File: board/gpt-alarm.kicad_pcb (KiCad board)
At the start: 2 copper layers, 105 x 64 mm, 12 parts, among them J1 Input, J2 Siren_Out, K1 HK19F-DCxxV-SHC, Q1 AO3400A, Q2 AO3400A

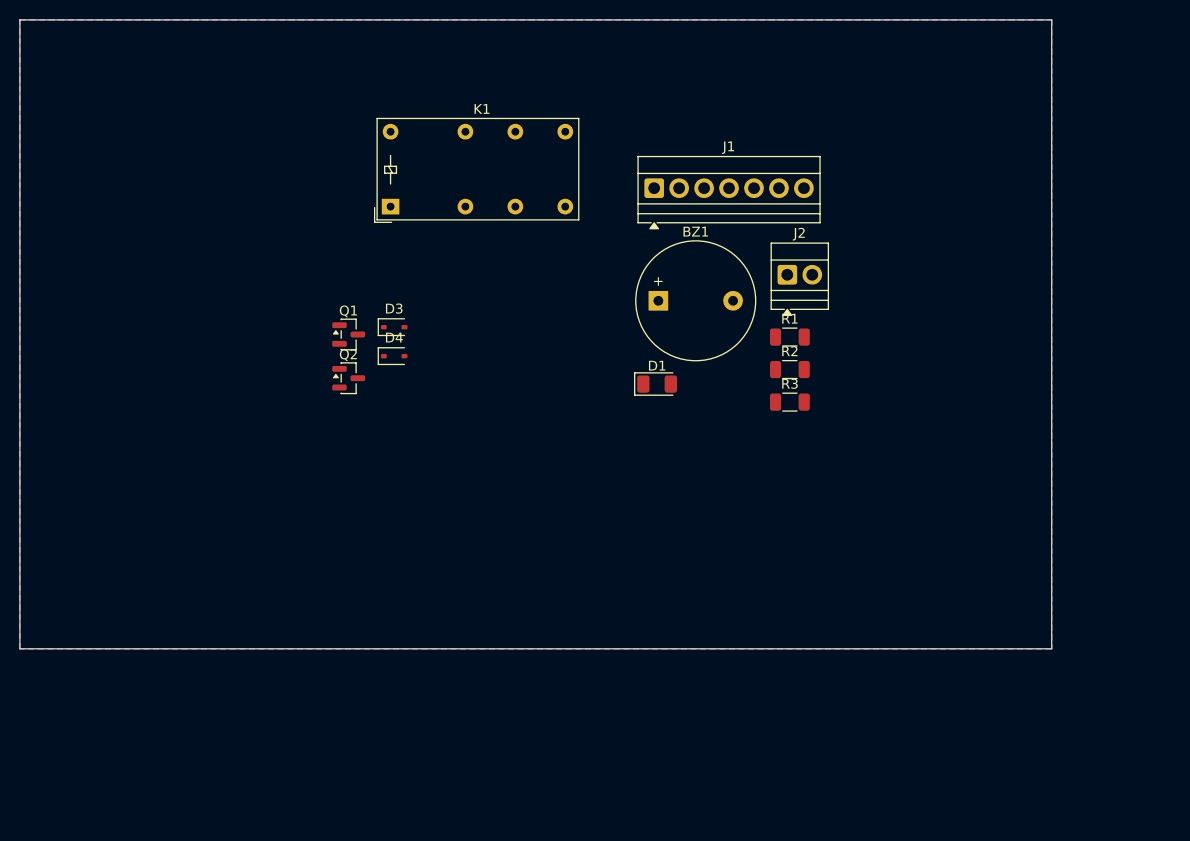
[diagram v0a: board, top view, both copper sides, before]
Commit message: feat: pcb layout
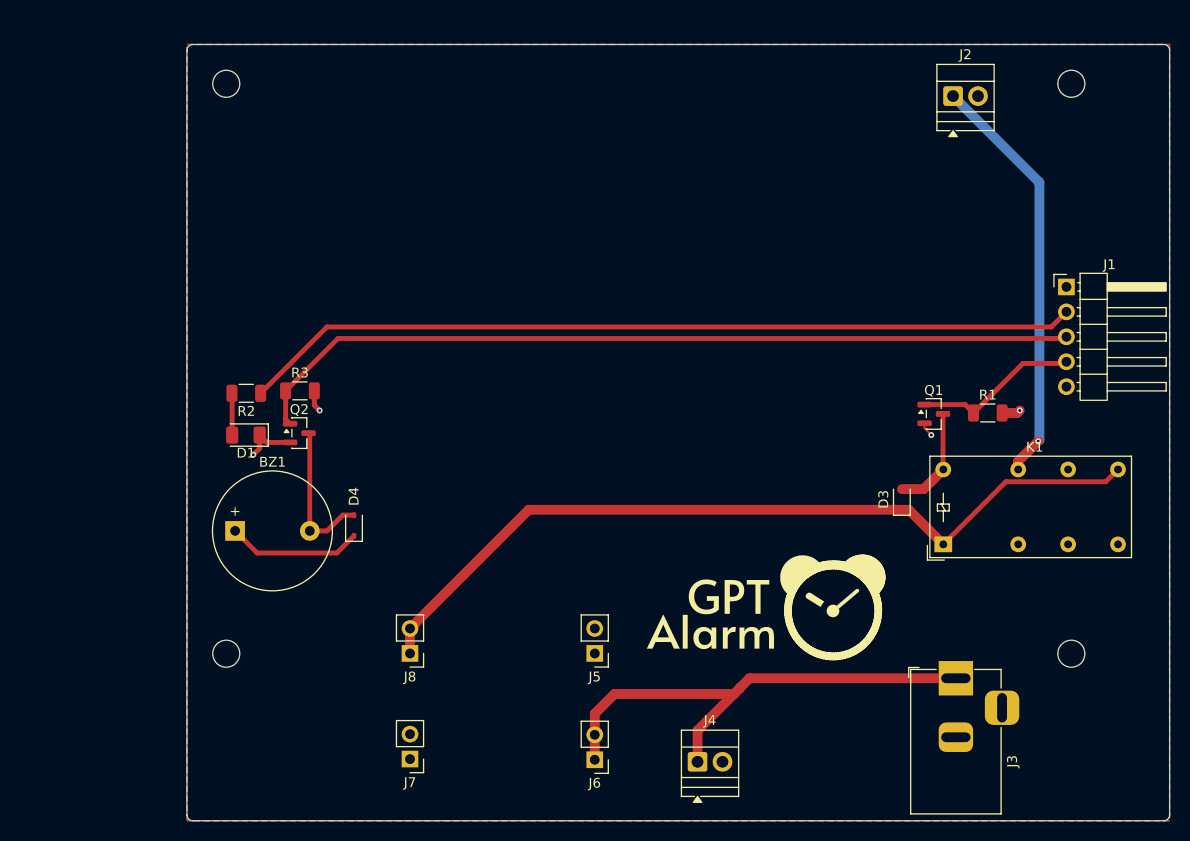
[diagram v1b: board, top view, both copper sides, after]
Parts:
- added J3: 19V IN, Connector_BarrelJack:BarrelJack_Horizontal, F.Cu at (181.8, 105.0)
- added J4: 19V OUT, TerminalBlock:TerminalBlock_Xinya_XY308-2.54-2P_1x02_P2.54mm_Horizontal, F.Cu at (155.5, 113.5)
- added J5: BUCK IN -, Connector_PinHeader_2.54mm:PinHeader_1x02_P2.54mm_Vertical, F.Cu at (145.0, 102.5)
- added J6: BUCK IN +, Connector_PinHeader_2.54mm:PinHeader_1x02_P2.54mm_Vertical, F.Cu at (145.0, 113.3)
- added J7: BUCK OUT -, Connector_PinHeader_2.54mm:PinHeader_1x02_P2.54mm_Vertical, F.Cu at (126.2, 113.2)
- added J8: BUCK OUT +, Connector_PinHeader_2.54mm:PinHeader_1x02_P2.54mm_Vertical, F.Cu at (126.2, 102.5)
- J1: value Input -> Conn_01x05_Pin; footprint TerminalBlock:TerminalBlock_Xinya_XY308-2.54-7P_1x07_P2.54mm_Horizontal -> Connector_PinHeader_2.54mm:PinHeader_1x05_P2.54mm_Horizontal
- moved K1 65.9 mm to (180.5, 91.4)
- moved Q1 60.1 mm to (179.5, 78.1)
- moved R2 55.4 mm to (109.5, 76.0), turned to 180 degrees
- moved D3 54.6 mm to (176.2, 86.8), turned to 90 degrees
- moved R3 49.9 mm to (115.0, 75.8)
- moved BZ1 49.0 mm to (108.4, 90.0)
- moved J1 43.1 mm to (193.0, 65.2)
- moved D1 42.2 mm to (109.5, 80.2), turned to 180 degrees
- moved J2 24.8 mm to (181.5, 45.8)
- moved R1 21.6 mm to (185.0, 78.0)
- moved D4 17.7 mm to (120.5, 89.5), turned to 90 degrees
- moved Q2 7.51 mm to (114.9, 80.0)
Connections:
- J1 pad 1: +12V -> GND
- J1 pad 2: +5V -> Net-(J1-Pin_2)
- J1 pad 3: +3V3 -> /buzz_sig
- J1 pad 5: /buzz_sig -> +5V
- R2 pad 1: Net-(J1-Pin_6) -> Net-(J1-Pin_2)
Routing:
- net Net-(J1-Pin_2): track 0.00 -> 85.6 mm
- net /buzz_sig: track 0.00 -> 85.2 mm
- net +12V: track 0.00 -> 84.2 mm
- net VCC: track 0.00 -> 51.4 mm
- net Net-(J2-Pin_1): track 0.00 -> 42.5 mm, vias 0 -> 1
- net Net-(J1-Pin_4): track 0.00 -> 16.9 mm
- net Net-(BZ1--): track 0.00 -> 15.2 mm
- net +5V: track 0.00 -> 13.8 mm
- net GND: track 0.00 -> 11.3 mm, vias 0 -> 4
- net Net-(D3-A): track 0.00 -> 10.7 mm
- net Net-(D1-A): track 0.00 -> 4.26 mm
- added copper zone on F.Cu, net +5V
- removed copper zone on F.Cu, net +12V
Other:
- board size 105 x 64 mm -> 100 x 79 mm
